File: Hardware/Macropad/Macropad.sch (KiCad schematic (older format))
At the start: 0 parts

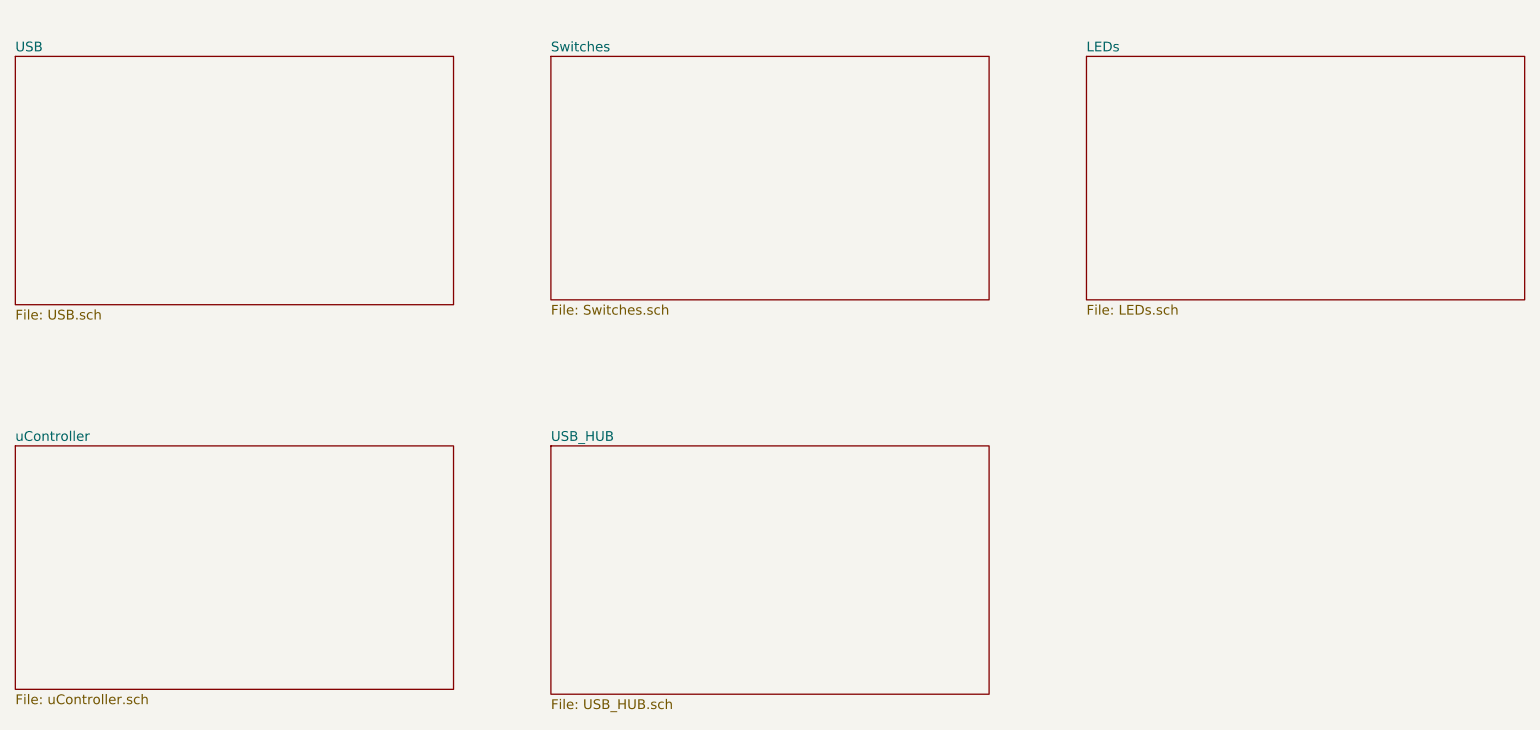
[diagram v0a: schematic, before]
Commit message: First pass of the layout done
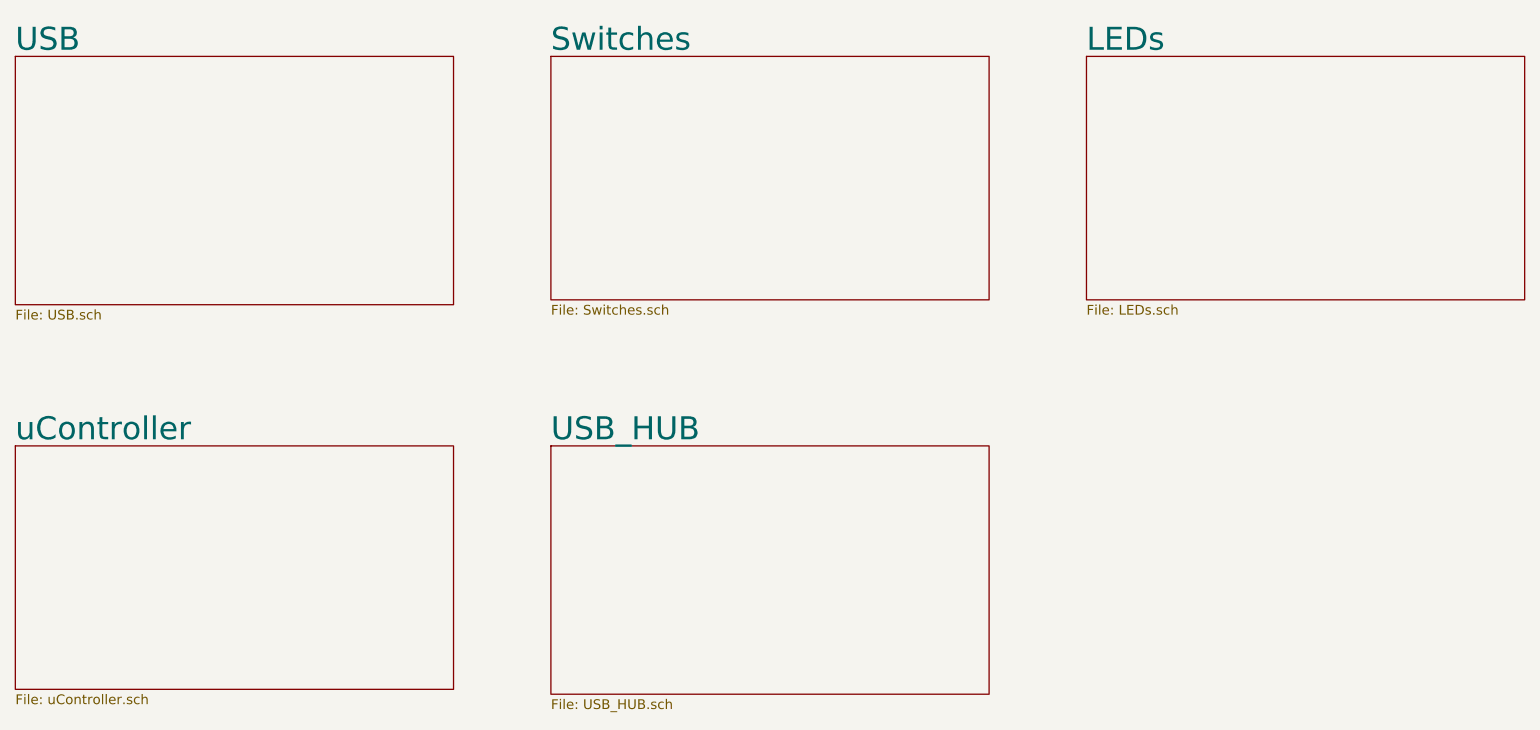
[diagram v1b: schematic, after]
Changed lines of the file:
@@
 S 1000 3000 2250 1275
 U 6114D32E
-F0 "USB" 50
+F0 "USB" 118
 F1 "USB.sch" 50
 $EndSheet
@@
 S 3750 3000 2250 1250
 U 61150193
-F0 "Switches" 50
+F0 "Switches" 118
 F1 "Switches.sch" 50
 $EndSheet
@@
 S 6500 3000 2250 1250
 U 61D5AB4C
-F0 "LEDs" 50
+F0 "LEDs" 118
 F1 "LEDs.sch" 50
 $EndSheet
@@
 S 1000 5000 2250 1250
 U 62022D96
-F0 "uController" 50
+F0 "uController" 118
 F1 "uController.sch" 50
 $EndSheet
@@
 S 3750 5000 2250 1275
 U 6247A5CE
-F0 "USB_HUB" 50
+F0 "USB_HUB" 118
 F1 "USB_HUB.sch" 50
 $EndSheet
